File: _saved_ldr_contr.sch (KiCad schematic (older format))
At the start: 15 parts, among them U1 ADG728, U2 ADG728, U3 ADG728, U5 LM317_3PinPackage

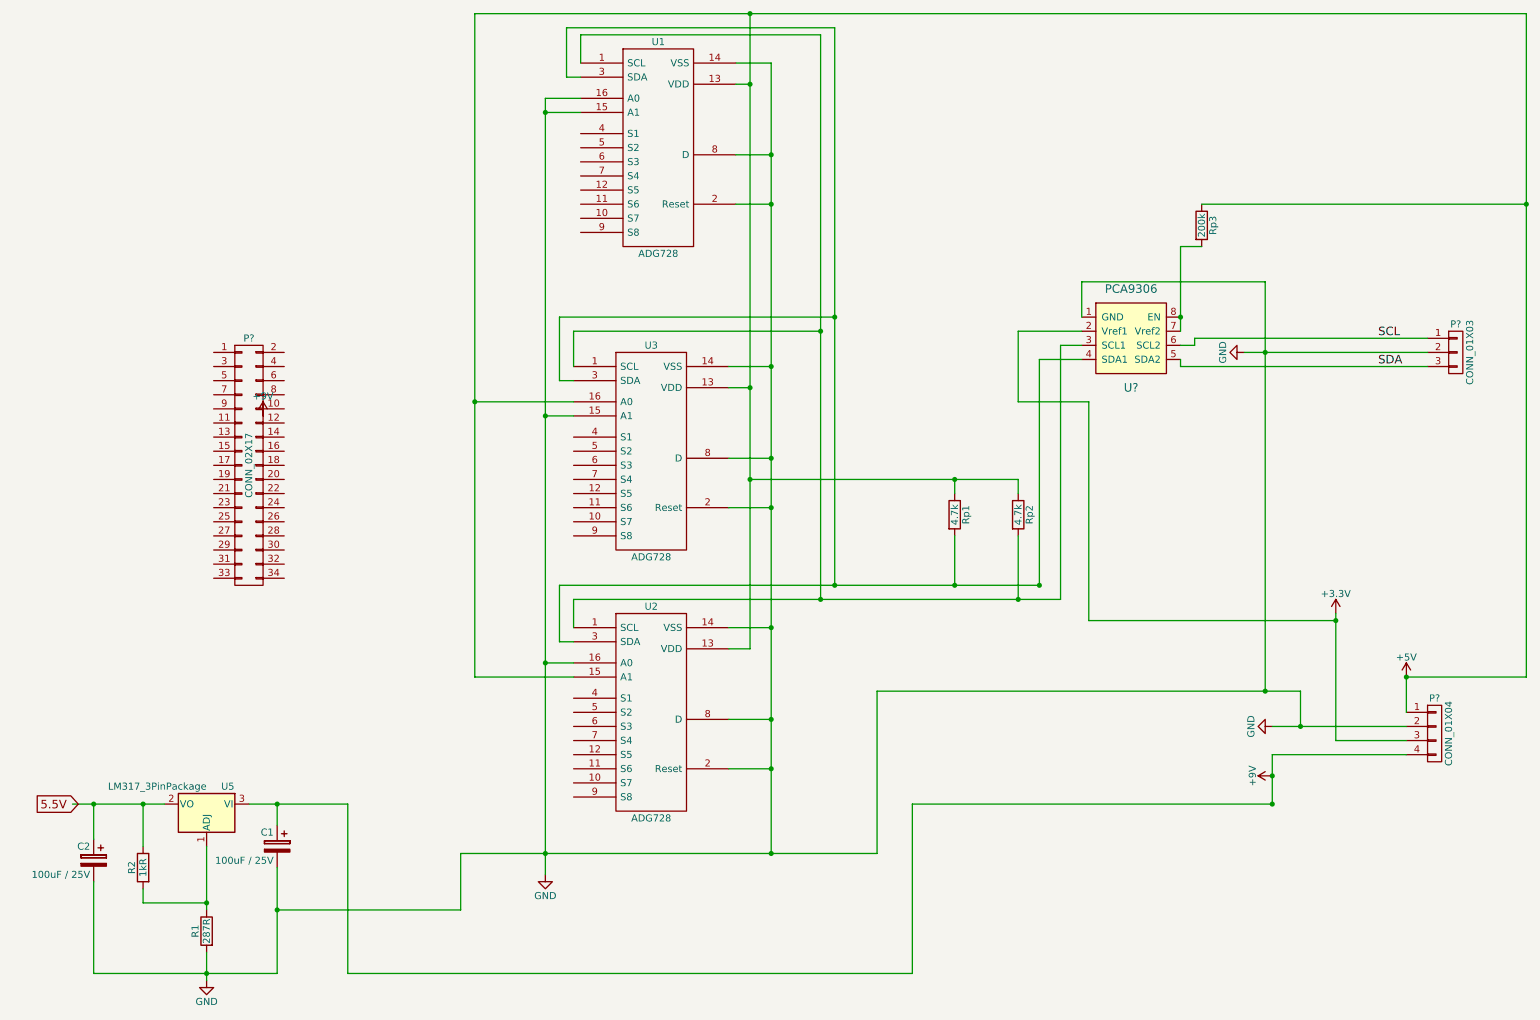
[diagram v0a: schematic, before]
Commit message: latest changes including pegel converter
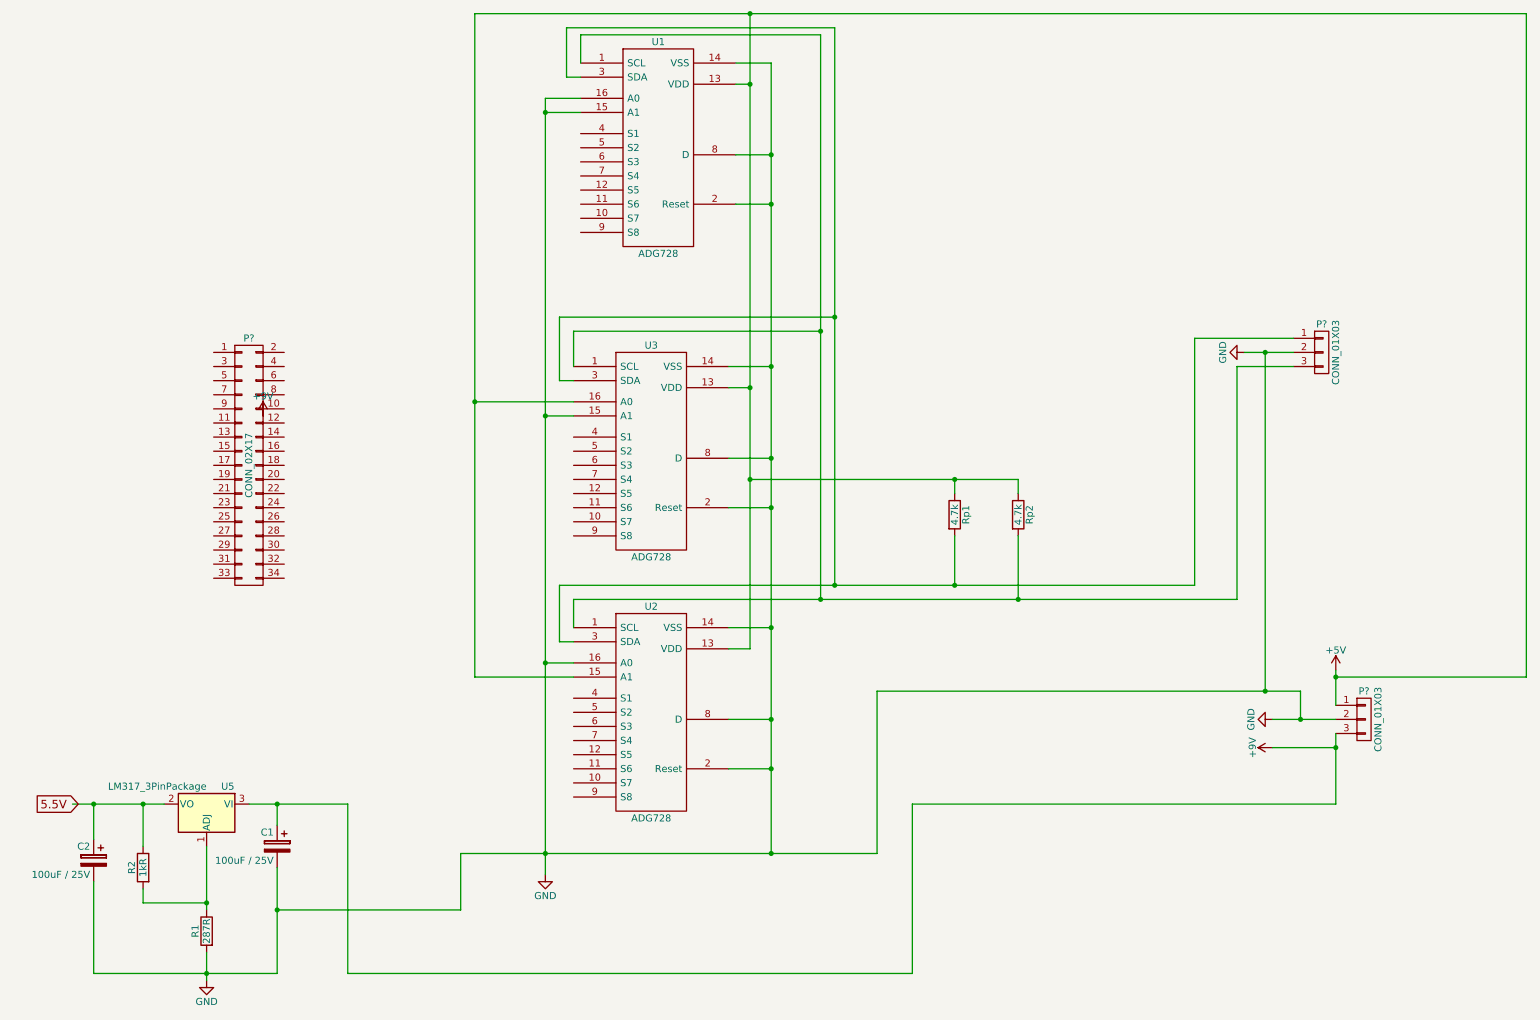
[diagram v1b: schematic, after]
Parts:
- removed P?: CONN_01X04, symbol CONN_01X04
- removed Rp3: 200k, symbol R
- removed U?: PCA9306, symbol PCA9306
- added P?: CONN_01X03, symbol CONN_01X03
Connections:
- net SCL is gone; now on an unnamed net: P?.1 (P1)
- net SDA is gone; now on an unnamed net: P?.3 (P3)
- net +5V: now also P?.1 (P1)
- net +9V: now also P?.3 (P3)
- net GND: now also P?.2 (P2)
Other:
- moved on the sheet: P?
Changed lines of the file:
@@
 LIBS:contrib
 LIBS:valves
-LIBS:ti
 LIBS:ldr_contr-cache
 EELAYER 25 0
@@
 $EndComp
 $Comp
-L +9V #PWR01
+L +9V #PWR?
 U 1 1 5ACA5CF6
 P 2100 3550
-F 0 "#PWR01" H 2100 3400 50  0001 C CNN
+F 0 "#PWR?" H 2100 3400 50  0001 C CNN
 F 1 "+9V" H 2100 3690 50  0000 C CNN
 F 2 "" H 2100 3550 50  0001 C CNN
@@
 $EndComp
 $Comp
-L GND #PWR02
+L GND #PWR?
 U 1 1 5ACA5D66
-P 9250 5750
-F 0 "#PWR02" H 9250 5500 50  0001 C CNN
-F 1 "GND" H 9250 5600 50  0000 C CNN
-F 2 "" H 9250 5750 50  0001 C CNN
-F 3 "" H 9250 5750 50  0001 C CNN
-	1    9250 5750
+P 9250 5700
+F 0 "#PWR?" H 9250 5450 50  0001 C CNN
+F 1 "GND" H 9250 5550 50  0000 C CNN
+F 2 "" H 9250 5700 50  0001 C CNN
+F 3 "" H 9250 5700 50  0001 C CNN
+	1    9250 5700
 	0    1    1    0
 $EndComp
 $Comp
-L GND #PWR03
+L GND #PWR?
 U 1 1 5ACA6104
 P 1700 7550
-F 0 "#PWR03" H 1700 7300 50  0001 C CNN
+F 0 "#PWR?" H 1700 7300 50  0001 C CNN
 F 1 "GND" H 1700 7400 50  0000 C CNN
 F 2 "" H 1700 7550 50  0001 C CNN
@@
 $EndComp
 $Comp
-L +9V #PWR04
+L +9V #PWR?
 U 1 1 5ACC57CF
-P 9250 6100
-F 0 "#PWR04" H 9250 5950 50  0001 C CNN
-F 1 "+9V" H 9250 6240 50  0000 C CNN
-F 2 "" H 9250 6100 50  0000 C CNN
-F 3 "" H 9250 6100 50  0000 C CNN
-	1    9250 6100
+P 9250 5900
+F 0 "#PWR?" H 9250 5750 50  0001 C CNN
+F 1 "+9V" H 9250 6040 50  0000 C CNN
+F 2 "" H 9250 5900 50  0000 C CNN
+F 3 "" H 9250 5900 50  0000 C CNN
+	1    9250 5900
 	0    -1   -1   0
 $EndComp
+$Comp
+L CONN_01X03 P?
+U 1 1 5ACC5819
+P 9900 5700
+F 0 "P?" H 9900 5900 50  0000 C CNN
+F 1 "CONN_01X03" V 10000 5700 50  0000 C CNN
+F 2 "" H 9900 5700 50  0000 C CNN
+F 3 "" H 9900 5700 50  0000 C CNN
+	1    9900 5700
+	1    0    0    -1
+$EndComp
 Wire Wire Line
 	2200 6450 2200 6300
 Wire Wire Line
+	9700 5800 9700 6300
+Wire Wire Line
+	9700 5900 9250 5900
+Wire Wire Line
+	9700 5700 9250 5700
+Connection ~ 9700 5900
+Wire Wire Line
 	2000 6300 2700 6300
 Wire Wire Line
@@
 Wire Wire Line
 	6700 7500 6700 6300
-$Comp
-L GND #PWR05
+Wire Wire Line
+	6700 6300 9700 6300
+$Comp
+L GND #PWR?
 U 1 1 5ACC5BA8
 P 4100 6800
-F 0 "#PWR05" H 4100 6550 50  0001 C CNN
+F 0 "#PWR?" H 4100 6550 50  0001 C CNN
 F 1 "GND" H 4100 6650 50  0000 C CNN
 F 2 "" H 4100 6800 50  0000 C CNN
@@
 L CONN_01X03 P?
 U 1 1 5ACC634F
-P 10550 3100
-F 0 "P?" H 10550 3300 50  0000 C CNN
-F 1 "CONN_01X03" V 10650 3100 50  0000 C CNN
-F 2 "" H 10550 3100 50  0000 C CNN
-F 3 "" H 10550 3100 50  0000 C CNN
-	1    10550 3100
-	1    0    0    -1
-$EndComp
-$Comp
-L GND #PWR06
+P 9600 3100
+F 0 "P?" H 9600 3300 50  0000 C CNN
+F 1 "CONN_01X03" V 9700 3100 50  0000 C CNN
+F 2 "" H 9600 3100 50  0000 C CNN
+F 3 "" H 9600 3100 50  0000 C CNN
+	1    9600 3100
+	1    0    0    -1
+$EndComp
+$Comp
+L GND #PWR?
 U 1 1 5ACC650F
 P 9050 3100
-F 0 "#PWR06" H 9050 2850 50  0001 C CNN
+F 0 "#PWR?" H 9050 2850 50  0001 C CNN
 F 1 "GND" H 9050 2950 50  0000 C CNN
 F 2 "" H 9050 3100 50  0000 C CNN
@@
 $EndComp
 Wire Wire Line
-	9050 3100 10350 3100
+	9050 3100 9400 3100
 Wire Wire Line
 	4300 5050 4300 4850
 Wire Wire Line
-	8600 3200 10350 3200
+	4300 4850 9000 4850
+Wire Wire Line
+	9000 4850 9000 3200
+Wire Wire Line
+	9000 3200 9400 3200
 Wire Wire Line
 	4300 5150 4200 5150
@@
 	4200 5150 4200 4750
 Wire Wire Line
-	8700 3000 10350 3000
+	4200 4750 8700 4750
+Wire Wire Line
+	8700 4750 8700 3000
+Wire Wire Line
+	8700 3000 9400 3000
 Wire Wire Line
 	4300 3200 4300 2950
@@
 Connection ~ 7000 4750
 Wire Wire Line
-	7450 4850 7450 4400
+	7450 4400 7450 4850
 Connection ~ 7450 4850
 Wire Wire Line
@@
 Connection ~ 7000 4000
 Wire Wire Line
-	9200 2600 9200 5500
+	9700 5600 9700 5350
+Wire Wire Line
+	9200 3100 9200 5500
 Wire Wire Line
 	6450 5500 9450 5500
+Wire Wire Line
+	9450 5500 9450 5700
+Connection ~ 9450 5700
 Connection ~ 9200 3100
 Wire Wire Line
@@
 Wire Wire Line
 	11050 700  11050 5400
+Wire Wire Line
+	11050 5400 9700 5400
+Connection ~ 9700 5400
 Connection ~ 5550 700
 $Comp
-L +5V #PWR07
+L +5V #PWR?
 U 1 1 5ACC87AF
-P 10200 5400
-F 0 "#PWR07" H 10200 5250 50  0001 C CNN
-F 1 "+5V" H 10200 5540 50  0000 C CNN
-F 2 "" H 10200 5400 50  0000 C CNN
-F 3 "" H 10200 5400 50  0000 C CNN
-	1    10200 5400
+P 9700 5350
+F 0 "#PWR?" H 9700 5200 50  0001 C CNN
+F 1 "+5V" H 9700 5490 50  0000 C CNN
+F 2 "" H 9700 5350 50  0000 C CNN
+F 3 "" H 9700 5350 50  0000 C CNN
+	1    9700 5350
 	1    0    0    -1
 $EndComp
 Wire Wire Line
 	3600 700  3600 5400
-$Comp
-L PCA9306 U?
-U 1 1 5ACC8C6F
-P 8250 2800
-F 0 "U?" H 8250 2250 60  0000 C CNN
-F 1 "PCA9306" H 8250 2950 60  0000 C CNN
-F 2 "" H 8150 2850 60  0000 C CNN
-F 3 "" H 8150 2850 60  0000 C CNN
-	1    8250 2800
-	1    0    0    -1
-$EndComp
-$Comp
-L CONN_01X04 P?
-U 1 1 5ACC8DCA
-P 10400 5800
-F 0 "P?" H 10400 6050 50  0000 C CNN
-F 1 "CONN_01X04" V 10500 5800 50  0000 C CNN
-F 2 "" H 10400 5800 50  0000 C CNN
-F 3 "" H 10400 5800 50  0000 C CNN
-	1    10400 5800
-	1    0    0    -1
-$EndComp
-Wire Wire Line
-	10200 5950 9250 5950
-Wire Wire Line
-	9250 5950 9250 6300
-Connection ~ 9250 6300
-Connection ~ 9250 6100
-Wire Wire Line
-	9250 6300 6700 6300
-Wire Wire Line
-	10200 5650 10200 5400
-Wire Wire Line
-	10200 5400 11050 5400
-Connection ~ 10200 5400
-Wire Wire Line
-	10200 5750 9250 5750
-Wire Wire Line
-	9450 5500 9450 5750
-Connection ~ 9450 5750
-$Comp
-L +3.3V #PWR08
-U 1 1 5ACC95B1
-P 9700 4950
-F 0 "#PWR08" H 9700 4800 50  0001 C CNN
-F 1 "+3.3V" H 9700 5090 50  0000 C CNN
-F 2 "" H 9700 4950 50  0000 C CNN
-F 3 "" H 9700 4950 50  0000 C CNN
-	1    9700 4950
-	1    0    0    -1
-$EndComp
-Wire Wire Line
-	10200 5850 9700 5850
-Wire Wire Line
-	9700 5850 9700 4950
-Wire Wire Line
-	7600 4750 7600 3150
-Wire Wire Line
-	7600 3150 7900 3150
-Connection ~ 7600 4750
-Wire Wire Line
-	4200 4750 7600 4750
-Wire Wire Line
-	4300 4850 7750 4850
-Wire Wire Line
-	7750 4850 7750 3050
-Wire Wire Line
-	7750 3050 7900 3050
-Wire Wire Line
-	8700 3000 8700 3050
-Wire Wire Line
-	8700 3050 8600 3050
-Wire Wire Line
-	8600 3200 8600 3150
-Wire Wire Line
-	9200 2600 7900 2600
-Wire Wire Line
-	7900 2600 7900 2850
-Wire Wire Line
-	9700 5000 7950 5000
-Wire Wire Line
-	7950 5000 7950 3450
-Wire Wire Line
-	7950 3450 7450 3450
-Wire Wire Line
-	7450 3450 7450 2950
-Wire Wire Line
-	7450 2950 7900 2950
-Connection ~ 9700 5000
-$Comp
-L R Rp3
-U 1 1 5ACC9DFB
-P 8750 2200
-F 0 "Rp3" V 8830 2200 50  0000 C CNN
-F 1 "200k" V 8750 2200 50  0000 C CNN
-F 2 "" V 8680 2200 50  0000 C CNN
-F 3 "" H 8750 2200 50  0000 C CNN
-	1    8750 2200
-	1    0    0    -1
-$EndComp
-Wire Wire Line
-	8600 2350 8600 2950
-Wire Wire Line
-	8600 2350 8750 2350
-Connection ~ 8600 2850
-Wire Wire Line
-	8750 2050 11050 2050
-Connection ~ 11050 2050
-Text Label 10000 3000 0    60   ~ 0
-SCL
-Text Label 10000 3200 0    60   ~ 0
-SDA
 $EndSCHEMATC
